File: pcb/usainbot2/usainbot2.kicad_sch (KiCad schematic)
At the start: 13 parts, among them J1 BT_MOD, J2 QTR1-L, J3 QTR1-R, J4 QTR8, J5 SWITCH, M1 Conn_01x02_Male, M2 Conn_01x02_Male, SW1 BTN1, SW2 BTN2

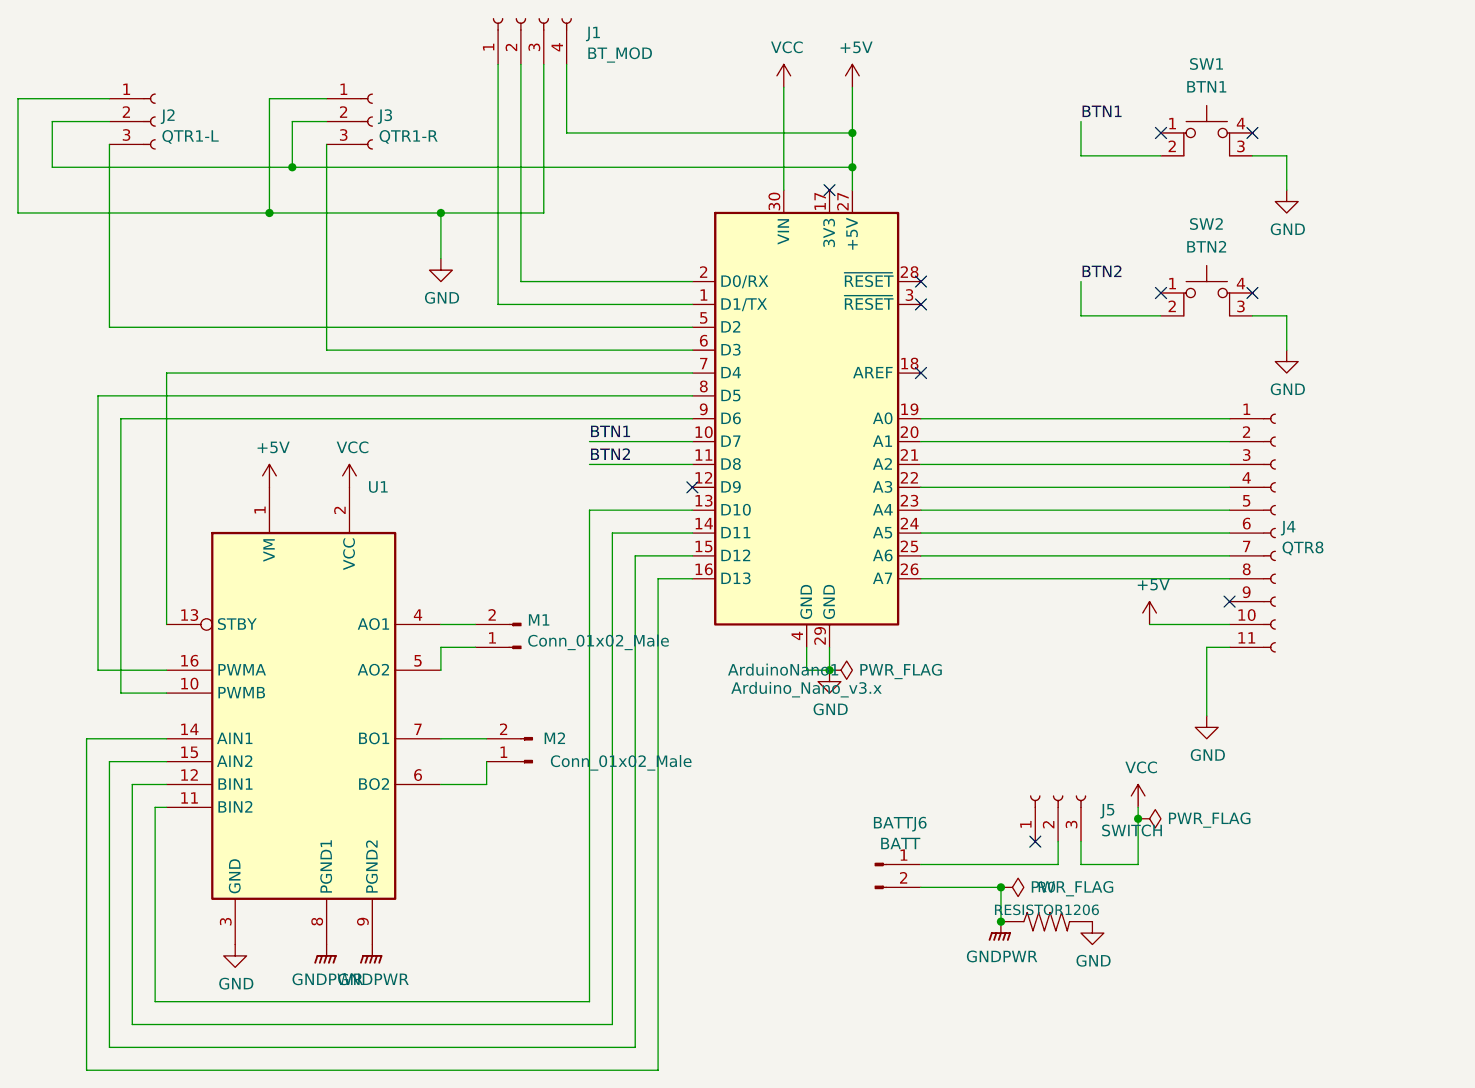
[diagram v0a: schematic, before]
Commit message: update pcb, falta rutear
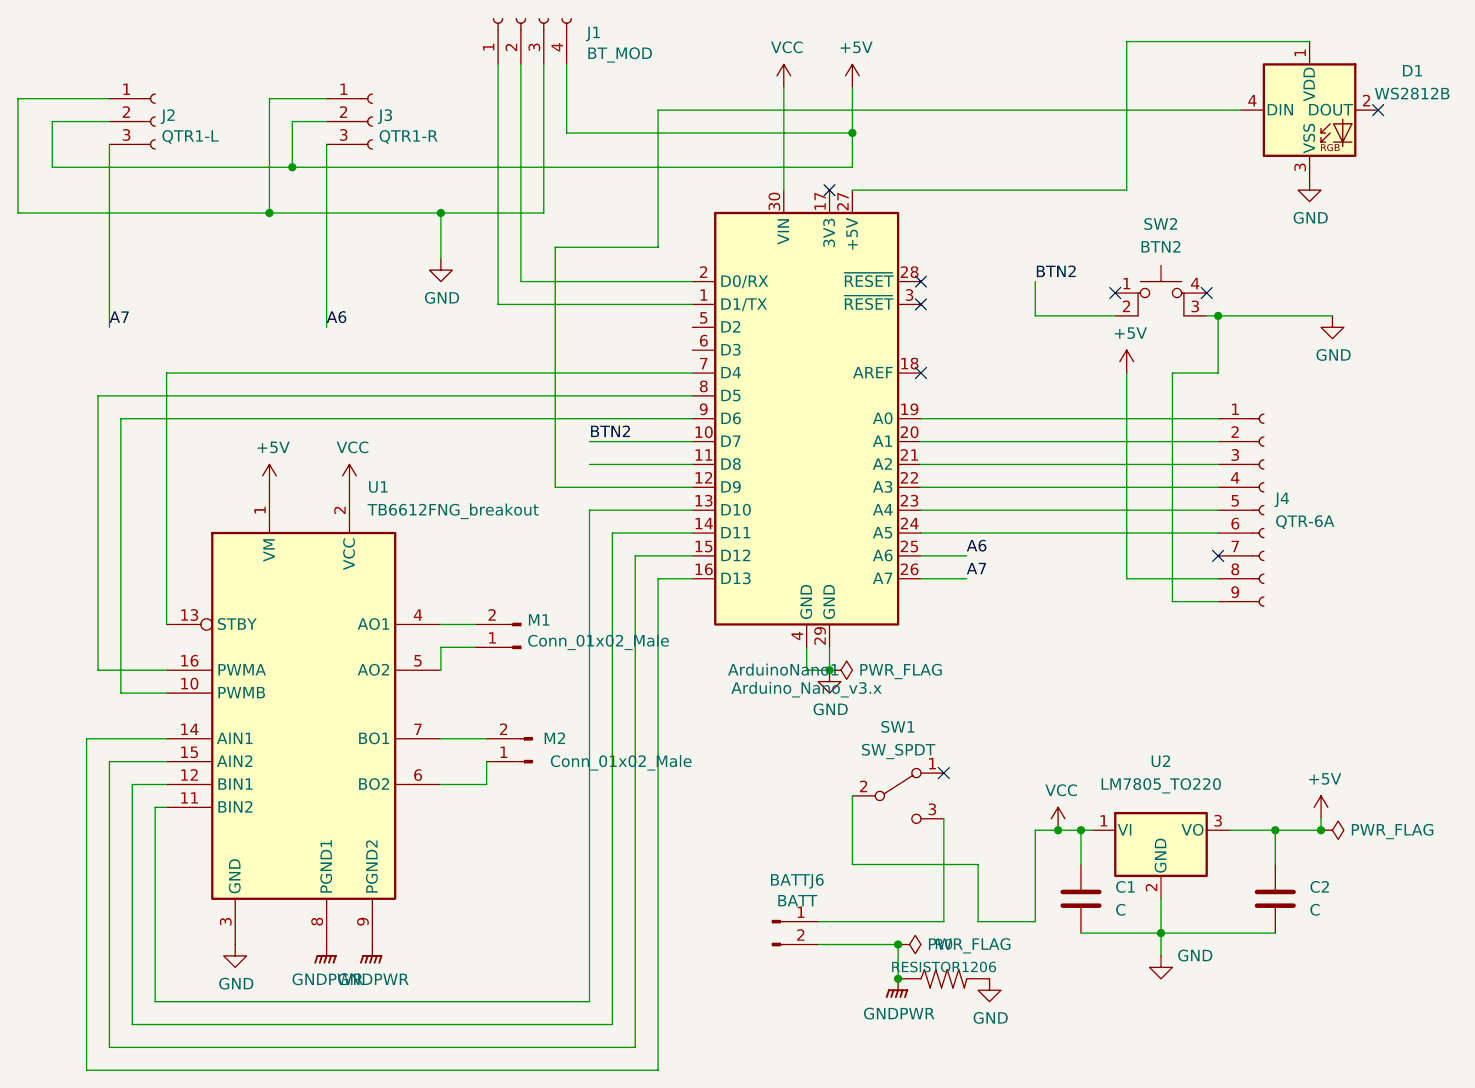
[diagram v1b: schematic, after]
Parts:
- removed J4: QTR8, Connector_PinSocket_2.54mm:PinSocket_1x11_P2.54mm_Horizontal, symbol usainbot2-rescue:Conn_01x11_Female-Connector
- removed J5: SWITCH, Connector_PinHeader_2.54mm:PinHeader_1x03_P2.54mm_Vertical, symbol usainbot2-rescue:Conn_01x03_Female-Connector
- removed SW1: BTN1, Button_Switch_THT:SW_PUSH_6mm, symbol Switch:SW_MEC_5E
- added C1, C2: C, Capacitor_SMD:C_0805_2012Metric_Pad1.18x1.45mm_HandSolder, symbol Device:C
- added D1: WS2812B, LED_SMD:LED_WS2812B_PLCC4_5.0x5.0mm_P3.2mm, symbol LED:WS2812B
- added J4: QTR-6A, Connector_PinHeader_2.54mm:PinHeader_1x09_P2.54mm_Horizontal, symbol Connector:Conn_01x09_Female
- added SW1: SW_SPDT, usainbot:TOGGLE_RA, symbol Switch:SW_SPDT
- added U2: LM7805_TO220, Package_TO_SOT_THT:TO-220-3_Vertical, symbol Regulator_Linear:LM7805_TO220
- BATTJ6: footprint Connector_PinHeader_2.54mm:PinHeader_1x02_P2.54mm_Horizontal -> Connector_Molex:Molex_KK-254_AE-6410-02A_1x02_P2.54mm_Vertical
- J2, J3: footprint Connector_PinHeader_2.54mm:PinHeader_1x03_P2.54mm_Vertical -> Connector_PinHeader_2.54mm:PinHeader_1x03_P2.54mm_Horizontal
- M1, M2: footprint Connector_PinHeader_2.54mm:PinHeader_1x02_P2.54mm_Horizontal -> Connector_PinHeader_2.54mm:PinHeader_1x02_P2.54mm_Vertical
- U1: value (none) -> TB6612FNG_breakout; footprint (none) -> usainbot:TB6612FNG Breakout
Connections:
- net BTN1 is gone; now on net BTN2: ArduinoNano1.10 (D7)
- net +5V: now also C2.1, J4.8 (Pin_8), U2.3 (VO); no longer ArduinoNano1.27 (+5V)
- net BTN2: no longer ArduinoNano1.11 (D8)
- net GND: now also C1.2, C2.2, D1.3 (VSS), J4.9 (Pin_9), U2.2 (GND)
- net VCC: now also C1.1, SW1.2 (B), U2.1 (VI)
- net at ArduinoNano1.12 (D9): now also D1.4 (DIN)
- net at ArduinoNano1.19 (A0): now also J4.1 (Pin_1)
- net at ArduinoNano1.20 (A1): now also J4.2 (Pin_2)
- net at ArduinoNano1.21 (A2): now also J4.3 (Pin_3)
- net at ArduinoNano1.22 (A3): now also J4.4 (Pin_4)
- net at ArduinoNano1.23 (A4): now also J4.5 (Pin_5)
- net at ArduinoNano1.24 (A5): now also J4.6 (Pin_6)
- net A6: now reaches ArduinoNano1.25 (A6)
- net A6: now also J3.3 (Pin_3)
- net A7: now reaches ArduinoNano1.26 (A7)
- net A7: now also J2.3 (Pin_3)
- net at ArduinoNano1.5 (D2): no longer J2.3 (Pin_3)
- net at ArduinoNano1.6 (D3): no longer J3.3 (Pin_3)
- net at BATTJ6.1 (Pin_1): now also SW1.3 (C)
- new net: ArduinoNano1.27 (+5V), D1.1 (VDD)
- no-connect marks 11 -> 9
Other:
- moved on the sheet: BATTJ6, R0, SW2
